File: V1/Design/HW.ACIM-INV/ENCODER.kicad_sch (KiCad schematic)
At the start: 25 parts, among them J8 ENCODER, Q2 60V/265mA, Q7 60V/265mA, Q8 60V/265mA, Q9 60V/265mA, U17 DIGI ISO 2-CH, U19 DIGI ISO 2-CH

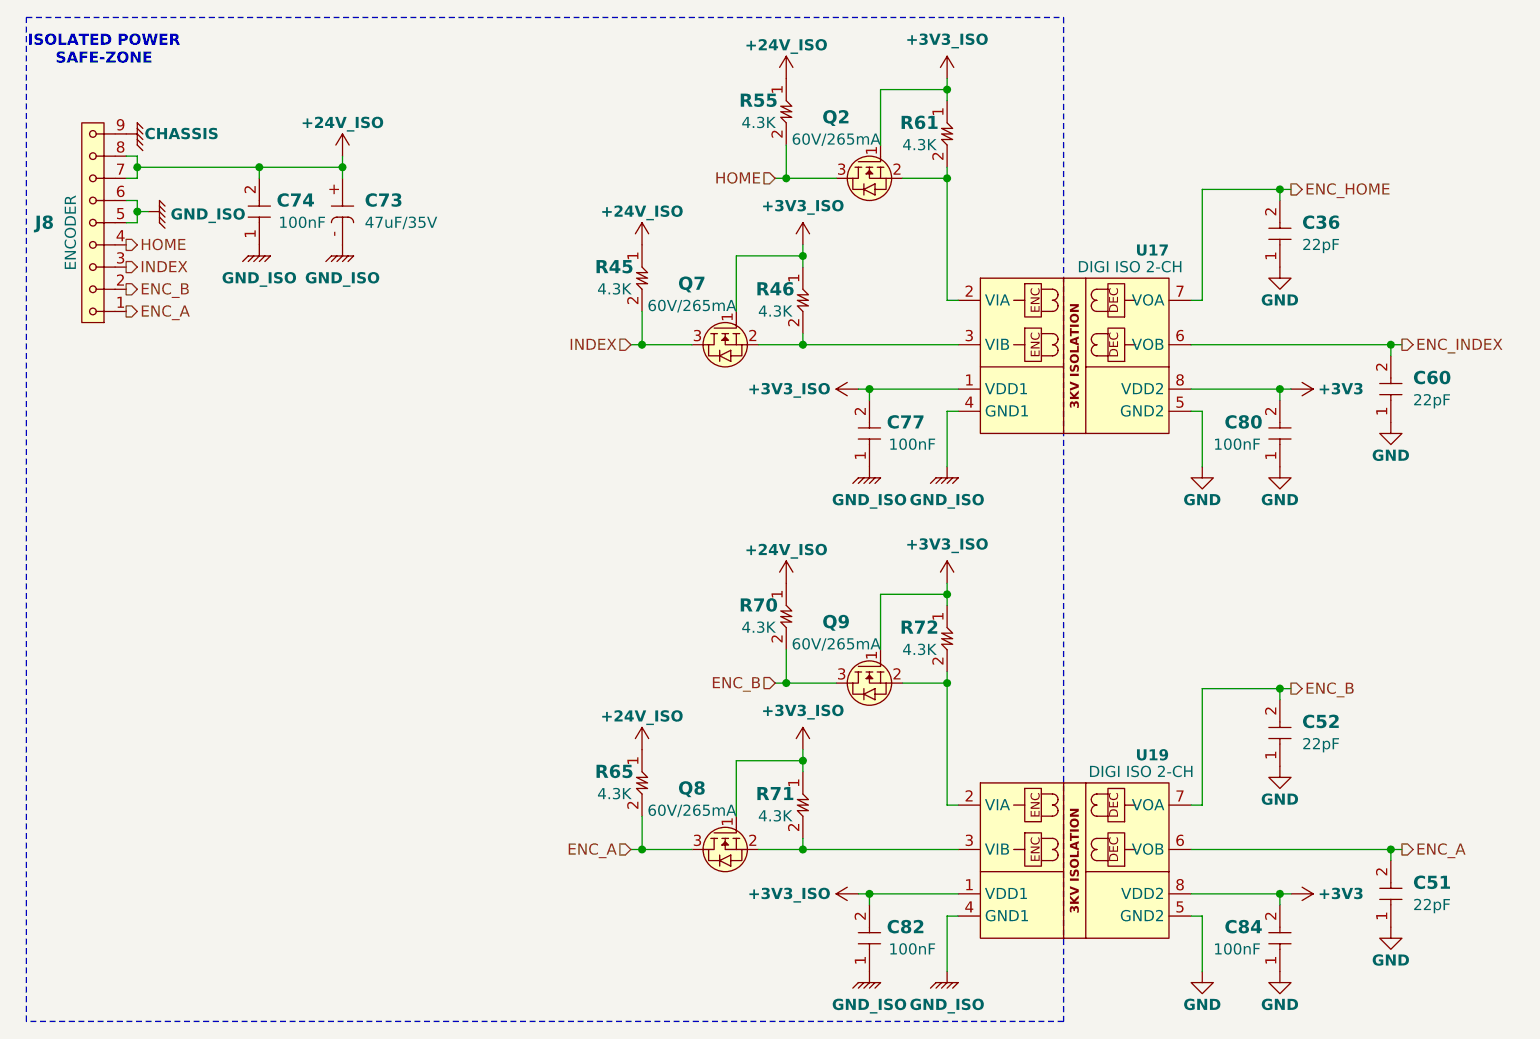
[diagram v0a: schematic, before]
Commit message: V1 schematic update 4
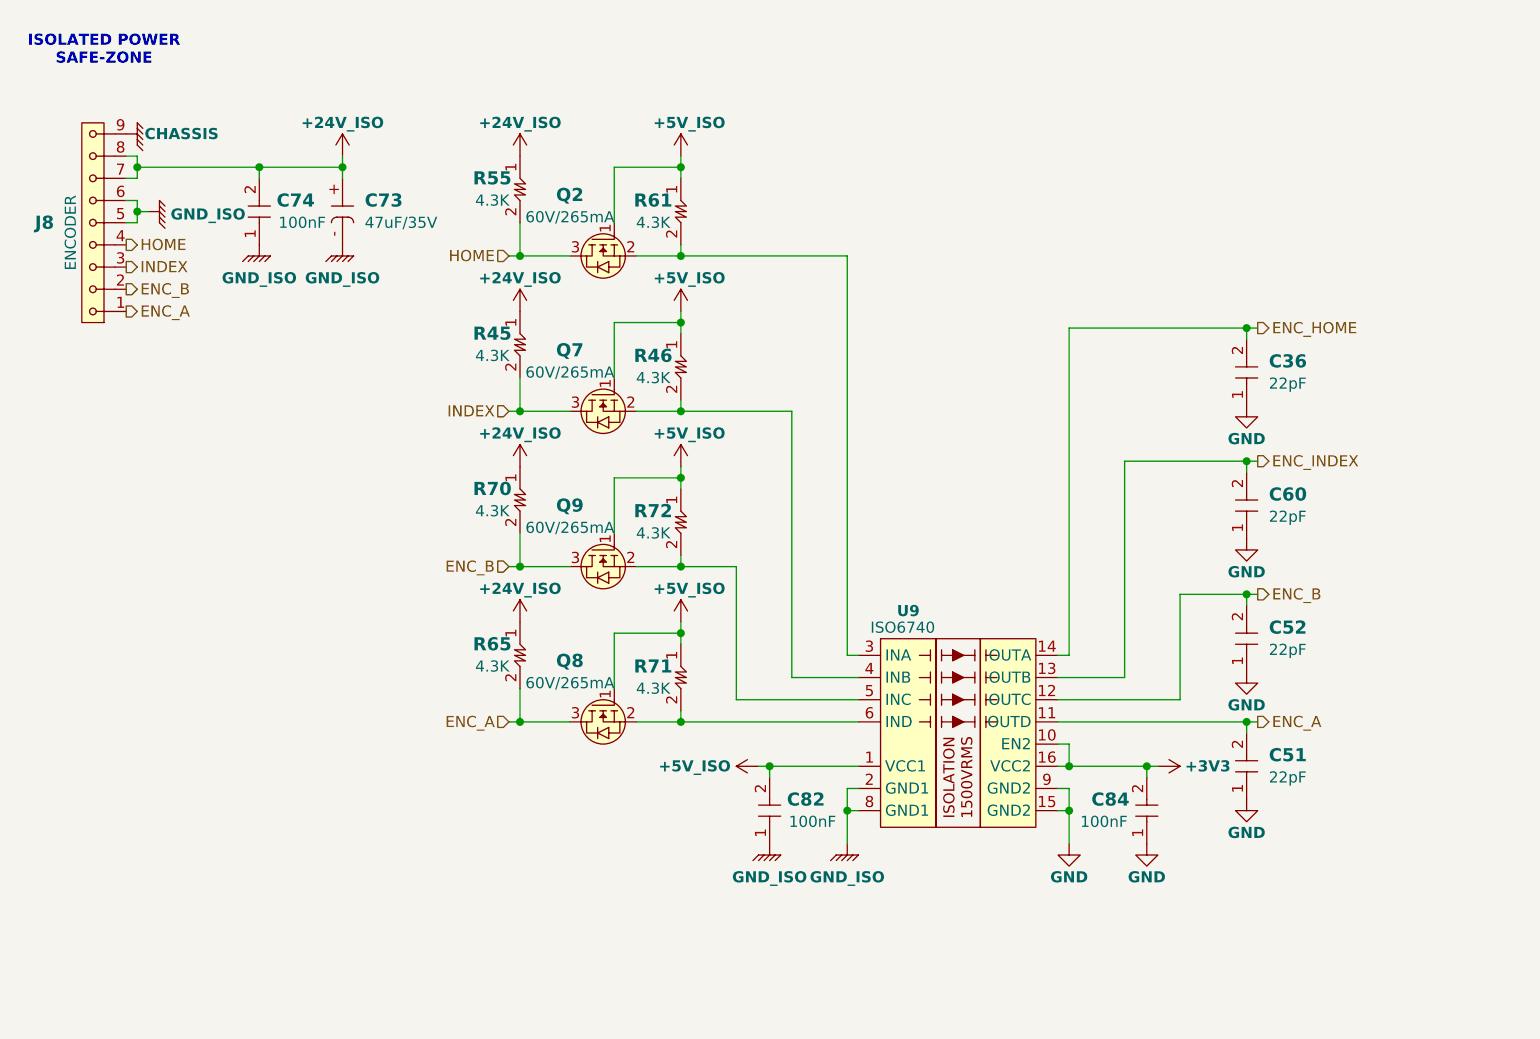
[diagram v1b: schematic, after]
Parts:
- removed C77, C80: 100nF, SAMPI:CAP0603, symbol SAMPI:CERCAP
- removed U17, U19: DIGI ISO 2-CH, SAMPI:SOIC8_ALL, symbol SAMPI:ADUM120N
- added U9: ISO6740, SAMPI:SOIC16-W, symbol SAMPI:ISO6740
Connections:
- net +3V3: now also U9.10 (EN2), U9.16 (VCC2)
- net ENC_A: now also U9.11 (OUTD)
- net ENC_B: now also U9.12 (OUTC)
- net ENC_HOME: now also U9.14 (OUTA)
- net ENC_INDEX: now also U9.13 (OUTB)
- net GND: now also U9.15 (GND2), U9.9 (GND2)
- net GND_ISO: now also U9.2 (GND1), U9.8 (GND1)
- net at Q2.2 (S), R61.2: now also U9.3 (INA)
- net at Q8.2 (S), R71.2: now also U9.6 (IND)
- net at Q7.2 (S), R46.2: now also U9.4 (INB)
- net at Q9.2 (S), R72.2: now also U9.5 (INC)
- net +3V3_ISO renamed +5V_ISO
- net +5V_ISO: now also U9.1 (VCC1)
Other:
- moved on the sheet: C36, C51, C52, C60, C82, C84, Q2, Q7, Q8, Q9, R45, R46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
